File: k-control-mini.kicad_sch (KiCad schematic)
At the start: 86 parts, among them J1_P1 IN_L, J1_P2 IN_GND, J1_P3 IN_R, J1_P4 OUT_R, J1_P5 OUT_GND, J1_P6 OUT_L, J2_P1 HP_R, J2_P2 HP_GND, J2_P3 HP_L, U1 H11L1S(TA)

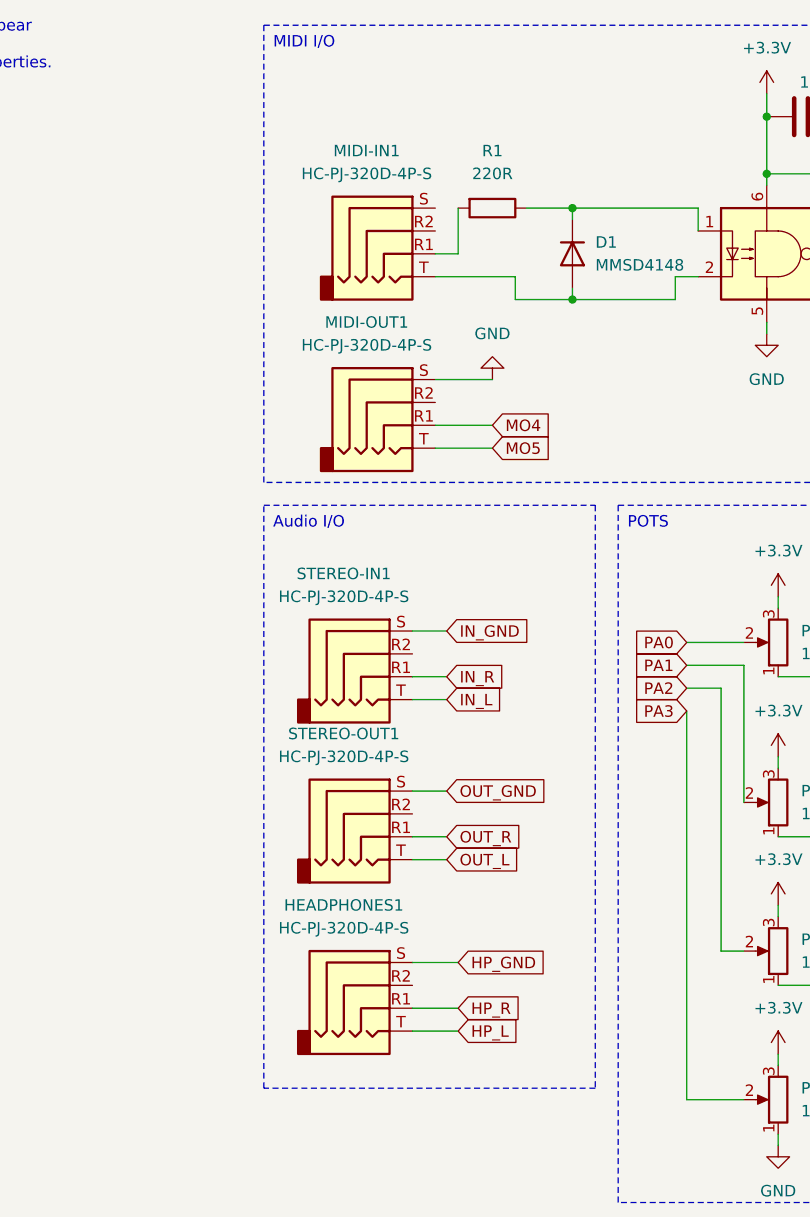
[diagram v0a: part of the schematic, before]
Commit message: thonk blue jacks
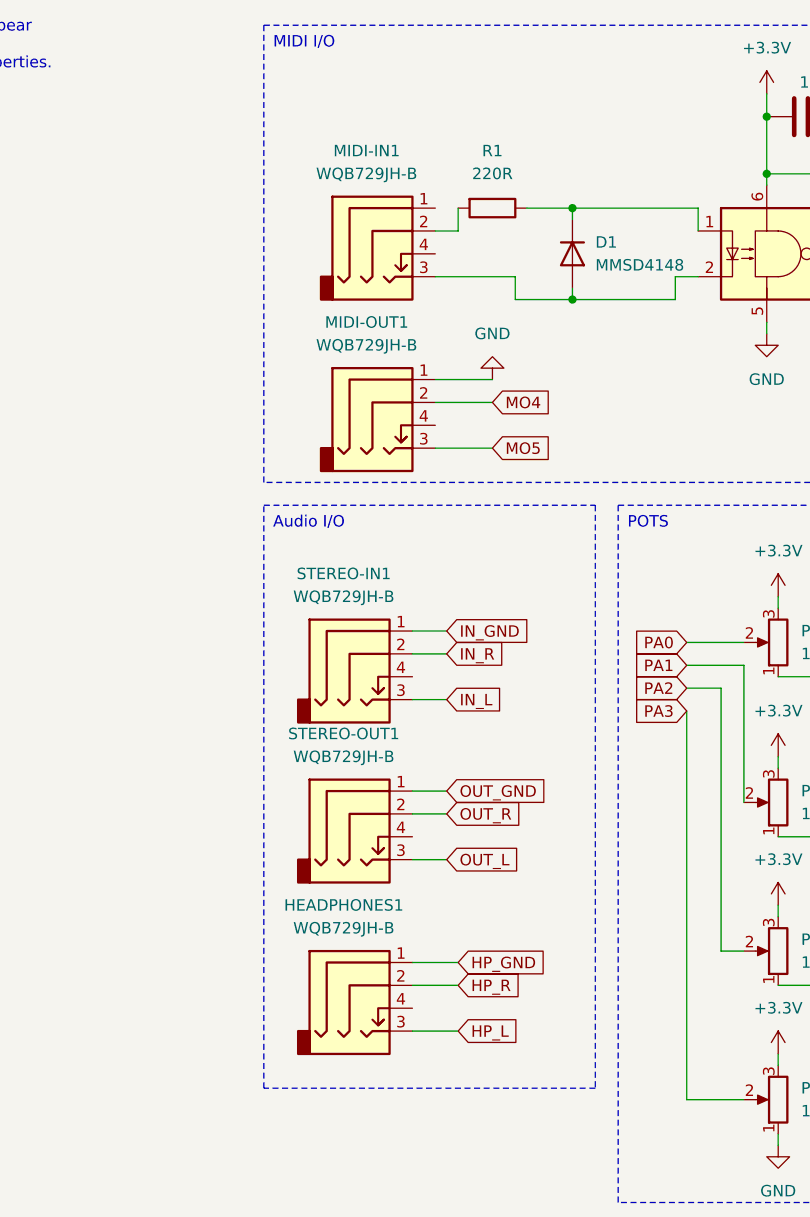
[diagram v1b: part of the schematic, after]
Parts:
- HEADPHONES1, MIDI-IN1, MIDI-OUT1, STEREO-IN1, STEREO-OUT1: value HC-PJ-320D-4P-S -> WQB729JH-B; footprint Connector_Audio:Jack_3.5mm_PJ320D_Horizontal -> Thonk:729JH-B; symbol Connector_Audio:AudioJack4 -> Thonk:729JH-B
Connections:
- net GND: now also MIDI-OUT1.1; no longer MIDI-OUT1.S
- net HP_GND: now also HEADPHONES1.1; no longer HEADPHONES1.S
- net HP_L: now also HEADPHONES1.3; no longer HEADPHONES1.T
- net HP_R: now also HEADPHONES1.2; no longer HEADPHONES1.R1
- net IN_GND: now also STEREO-IN1.1; no longer STEREO-IN1.S
- net IN_L: now also STEREO-IN1.3; no longer STEREO-IN1.T
- net IN_R: now also STEREO-IN1.2; no longer STEREO-IN1.R1
- net MO4: now also MIDI-OUT1.2; no longer MIDI-OUT1.R1
- net MO5: now also MIDI-OUT1.3; no longer MIDI-OUT1.T
- net OUT_GND: now also STEREO-OUT1.1; no longer STEREO-OUT1.S
- net OUT_L: now also STEREO-OUT1.3; no longer STEREO-OUT1.T
- net OUT_R: now also STEREO-OUT1.2; no longer STEREO-OUT1.R1
- net at R1.2: now also MIDI-IN1.2; no longer MIDI-IN1.R1
- net at D1.2 (A), U1.2: now also MIDI-IN1.3; no longer MIDI-IN1.T
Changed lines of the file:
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@@
     (stroke (width 0) (type default))
   )
-  (wire (pts (xy 38.1 45.72) (xy 38.1 40.64))
-    (stroke (width 0) (type default))
-  )
   (wire (pts (xy 50.8 41.91) (xy 50.8 40.64))
     (stroke (width 0) (type default))
@@
     (stroke (width 0) (type default))
   )
+  (wire (pts (xy 33.02 107.95) (xy 36.83 107.95))
+    (stroke (width 0) (type default))
+  )
   (wire (pts (xy 195.58 40.64) (xy 195.58 49.53))
     (stroke (width 0) (type default))
@@
     (stroke (width 0) (type default))
   )
+  (wire (pts (xy 35.56 43.18) (xy 38.1 43.18))
+    (stroke (width 0) (type default))
+  )
   (wire (pts (xy 73.66 127) (xy 78.74 127))
     (stroke (width 0) (type default))
   )
+  (wire (pts (xy 35.56 62.23) (xy 41.91 62.23))
+    (stroke (width 0) (type default))
+  )
   (wire (pts (xy 63.5 93.98) (xy 67.31 93.98))
     (stroke (width 0) (type default))
@@
     (stroke (width 0) (type default))
   )
-  (wire (pts (xy 35.56 45.72) (xy 38.1 45.72))
-    (stroke (width 0) (type default))
-  )
   (wire (pts (xy 33.02 105.41) (xy 36.83 105.41))
     (stroke (width 0) (type default))
@@
     (stroke (width 0) (type default))
   )
-  (wire (pts (xy 222.25 123.19) (xy 201.93 123.19))
+  (wire (pts (xy 33.02 127) (xy 38.1 127))
     (stroke (width 0) (type default))
   )
-  (wire (pts (xy 33.02 92.71) (xy 36.83 92.71))
+  (wire (pts (xy 222.25 123.19) (xy 201.93 123.19))
     (stroke (width 0) (type default))
   )
@@
     (stroke (width 0) (type default))
   )
+  (wire (pts (xy 38.1 43.18) (xy 38.1 40.64))
+    (stroke (width 0) (type default))
+  )
   (wire (pts (xy 62.23 48.26) (xy 64.77 48.26))
     (stroke (width 0) (type default))
@@
     (stroke (width 0) (type default))
   )
-  (wire (pts (xy 35.56 64.77) (xy 41.91 64.77))
-    (stroke (width 0) (type default))
-  )
   (wire (pts (xy 215.9 115.57) (xy 222.25 115.57))
     (stroke (width 0) (type default))
@@
     (stroke (width 0) (type default))
   )
-  (wire (pts (xy 33.02 110.49) (xy 36.83 110.49))
-    (stroke (width 0) (type default))
-  )
   (wire (pts (xy 234.95 135.89) (xy 241.3 135.89))
     (stroke (width 0) (type default))
@@
     (stroke (width 0) (type default))
   )
+  (wire (pts (xy 33.02 90.17) (xy 36.83 90.17))
+    (stroke (width 0) (type default))
+  )
   (polyline (pts (xy 224.79 125.73) (xy 232.41 125.73))
     (stroke (width 0) (type solid))
@@
     (stroke (width 0) (type default))
   )
-  (wire (pts (xy 33.02 129.54) (xy 38.1 129.54))
-    (stroke (width 0) (type default))
-  )
   (image (at -43.18 124.46)
     (data
@@
     )
   )
-  (global_label "IN_R" (shape input) (at 36.83 92.71 0) (fields_autoplaced)
+  (global_label "IN_R" (shape input) (at 36.83 90.17 0) (fields_autoplaced)
     (effects (font (size 1.27 1.27)) (justify left))
-    (property "Intersheetrefs" "${INTERSHEET_REFS}" (at 43.9881 92.71 0)
+    (property "Intersheetrefs" "${INTERSHEET_REFS}" (at 43.9881 90.17 0)
       (effects (font (size 1.27 1.27)) (justify left) hide)
     )
@@
     )
   )
-  (global_label "MO4" (shape input) (at 41.91 64.77 0) (fields_autoplaced)
+  (global_label "MO4" (shape input) (at 41.91 62.23 0) (fields_autoplaced)
     (effects (font (size 1.27 1.27)) (justify left))
-    (property "Intersheetrefs" "${INTERSHEET_REFS}" (at 48.3145 64.6906 0)
+    (property "Intersheetrefs" "${INTERSHEET_REFS}" (at 48.3145 62.1506 0)
       (effects (font (size 1.27 1.27)) (justify left) hide)
     )
@@
     )
   )
-  (global_label "HP_R" (shape input) (at 38.1 129.54 0) (fields_autoplaced)
+  (global_label "HP_R" (shape input) (at 38.1 127 0) (fields_autoplaced)
     (effects (font (size 1.27 1.27)) (justify left))
-    (property "Intersheetrefs" "${INTERSHEET_REFS}" (at 45.3512 129.4606 0)
+    (property "Intersheetrefs" "${INTERSHEET_REFS}" (at 45.3512 126.9206 0)
       (effects (font (size 1.27 1.27)) (justify left) hide)
     )
@@
     )
   )
-  (global_label "OUT_R" (shape input) (at 36.83 110.49 0) (fields_autoplaced)
+  (global_label "OUT_R" (shape input) (at 36.83 107.95 0) (fields_autoplaced)
     (effects (font (size 1.27 1.27)) (justify left))
-    (property "Intersheetrefs" "${INTERSHEET_REFS}" (at 45.6814 110.49 0)
+    (property "Intersheetrefs" "${INTERSHEET_REFS}" (at 45.6814 107.95 0)
       (effects (font (size 1.27 1.27)) (justify left) hide)
     )
@@
     )
   )
-  (symbol (lib_id "Connector_Audio:AudioJack4") (at 30.48 43.18 0) (unit 1)
+  (symbol (lib_id "Thonk:729JH-B") (at 30.48 43.18 0) (unit 1)
     (in_bom yes) (on_board yes) (dnp no) (fields_autoplaced)
     (property "Reference" "MIDI-IN1" (at 27.94 34.29 0)
       (effects (font (size 1.27 1.27)))
     )
-    (property "Value" "HC-PJ-320D-4P-S" (at 27.94 36.83 0)
+    (property "Value" "WQB729JH-B" (at 27.94 36.83 0)
       (effects (font (size 1.27 1.27)))
     )
-    (property "Footprint" "Connector_Audio:Jack_3.5mm_PJ320D_Horizontal" (at 30.48 43.18 0)
+    (property "Footprint" "Thonk:729JH-B" (at 29.21 52.07 0)
       (effects (font (size 1.27 1.27)) hide)
     )
-    (property "Datasheet" "~" (at 30.48 43.18 0)
+    (property "Datasheet" "https://www.thonk.co.uk/wp-content/uploads/2022/11/WQP729JH-datasheet.jpg" (at 33.02 54.61 0)
       (effects (font (size 1.27 1.27)) hide)
     )
-    (pin "S")
-    (pin "R1")
-    (pin "T")
-    (pin "R2")
+    (pin "1")
+    (pin "2")
+    (pin "4")
+    (pin "3")
     (instances
       (project "k-control-mini"
@@
     )
   )
-  (symbol (lib_id "Connector_Audio:AudioJack4") (at 27.94 90.17 0) (unit 1)
+  (symbol (lib_id "Thonk:729JH-B") (at 27.94 90.17 0) (unit 1)
     (in_bom yes) (on_board yes) (dnp no) (fields_autoplaced)
     (property "Reference" "STEREO-IN1" (at 25.4 81.28 0)
       (effects (font (size 1.27 1.27)))
     )
-    (property "Value" "HC-PJ-320D-4P-S" (at 25.4 83.82 0)
+    (property "Value" "WQB729JH-B" (at 25.4 83.82 0)
       (effects (font (size 1.27 1.27)))
     )
-    (property "Footprint" "Connector_Audio:Jack_3.5mm_PJ320D_Horizontal" (at 27.94 90.17 0)
+    (property "Footprint" "Thonk:729JH-B" (at 26.67 99.06 0)
       (effects (font (size 1.27 1.27)) hide)
     )
-    (property "Datasheet" "~" (at 27.94 90.17 0)
+    (property "Datasheet" "https://www.thonk.co.uk/wp-content/uploads/2022/11/WQP729JH-datasheet.jpg" (at 30.48 101.6 0)
       (effects (font (size 1.27 1.27)) hide)
     )
-    (pin "S")
-    (pin "R1")
-    (pin "T")
-    (pin "R2")
+    (pin "2")
+    (pin "4")
+    (pin "3")
+    (pin "1")
     (instances
       (project "k-control-mini"
@@
     )
   )
-  (symbol (lib_id "Connector_Audio:AudioJack4") (at 30.48 62.23 0) (unit 1)
+  (symbol (lib_id "Thonk:729JH-B") (at 30.48 62.23 0) (unit 1)
     (in_bom yes) (on_board yes) (dnp no) (fields_autoplaced)
     (property "Reference" "MIDI-OUT1" (at 27.94 53.34 0)
       (effects (font (size 1.27 1.27)))
     )
-    (property "Value" "HC-PJ-320D-4P-S" (at 27.94 55.88 0)
+    (property "Value" "WQB729JH-B" (at 27.94 55.88 0)
       (effects (font (size 1.27 1.27)))
     )
-    (property "Footprint" "Connector_Audio:Jack_3.5mm_PJ320D_Horizontal" (at 30.48 62.23 0)
+    (property "Footprint" "Thonk:729JH-B" (at 29.21 71.12 0)
       (effects (font (size 1.27 1.27)) hide)
     )
-    (property "Datasheet" "~" (at 30.48 62.23 0)
+    (property "Datasheet" "https://www.thonk.co.uk/wp-content/uploads/2022/11/WQP729JH-datasheet.jpg" (at 33.02 73.66 0)
       (effects (font (size 1.27 1.27)) hide)
     )
-    (pin "S")
-    (pin "R1")
-    (pin "T")
-    (pin "R2")
+    (pin "1")
+    (pin "2")
+    (pin "3")
+    (pin "4")
     (instances
       (project "k-control-mini"
@@
     )
   )
-  (symbol (lib_id "Connector_Audio:AudioJack4") (at 27.94 107.95 0) (unit 1)
+  (symbol (lib_id "Thonk:729JH-B") (at 27.94 107.95 0) (unit 1)
     (in_bom yes) (on_board yes) (dnp no) (fields_autoplaced)
     (property "Reference" "STEREO-OUT1" (at 25.4 99.06 0)
       (effects (font (size 1.27 1.27)))
     )
-    (property "Value" "HC-PJ-320D-4P-S" (at 25.4 101.6 0)
+    (property "Value" "WQB729JH-B" (at 25.4 101.6 0)
       (effects (font (size 1.27 1.27)))
     )
-    (property "Footprint" "Connector_Audio:Jack_3.5mm_PJ320D_Horizontal" (at 27.94 107.95 0)
+    (property "Footprint" "Thonk:729JH-B" (at 26.67 116.84 0)
       (effects (font (size 1.27 1.27)) hide)
     )
-    (property "Datasheet" "~" (at 27.94 107.95 0)
+    (property "Datasheet" "https://www.thonk.co.uk/wp-content/uploads/2022/11/WQP729JH-datasheet.jpg" (at 30.48 119.38 0)
       (effects (font (size 1.27 1.27)) hide)
     )
-    (pin "S")
-    (pin "R1")
-    (pin "T")
-    (pin "R2")
+    (pin "1")
+    (pin "3")
+    (pin "4")
+    (pin "2")
     (instances
       (project "k-control-mini"
@@
     )
   )
-  (symbol (lib_id "Connector_Audio:AudioJack4") (at 27.94 127 0) (unit 1)
+  (symbol (lib_id "Thonk:729JH-B") (at 27.94 127 0) (unit 1)
     (in_bom yes) (on_board yes) (dnp no) (fields_autoplaced)
     (property "Reference" "HEADPHONES1" (at 25.4 118.11 0)
       (effects (font (size 1.27 1.27)))
     )
-    (property "Value" "HC-PJ-320D-4P-S" (at 25.4 120.65 0)
+    (property "Value" "WQB729JH-B" (at 25.4 120.65 0)
       (effects (font (size 1.27 1.27)))
     )
-    (property "Footprint" "Connector_Audio:Jack_3.5mm_PJ320D_Horizontal" (at 27.94 127 0)
+    (property "Footprint" "Thonk:729JH-B" (at 26.67 135.89 0)
       (effects (font (size 1.27 1.27)) hide)
     )
-    (property "Datasheet" "~" (at 27.94 127 0)
+    (property "Datasheet" "https://www.thonk.co.uk/wp-content/uploads/2022/11/WQP729JH-datasheet.jpg" (at 30.48 138.43 0)
       (effects (font (size 1.27 1.27)) hide)
     )
-    (pin "S")
-    (pin "R2")
-    (pin "T")
-    (pin "R1")
+    (pin "3")
+    (pin "1")
+    (pin "4")
+    (pin "2")
     (instances
       (project "k-control-mini"
